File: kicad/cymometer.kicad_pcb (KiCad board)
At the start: 2 copper layers, 88.4 x 62 mm, 41 parts, among them IC1 ATTINY2313-P, P1 BNC, P2 CONN_2, P3 CONN_3X2, P4 CONN_12, Q1 BC550, U1 7805, X1 16.000

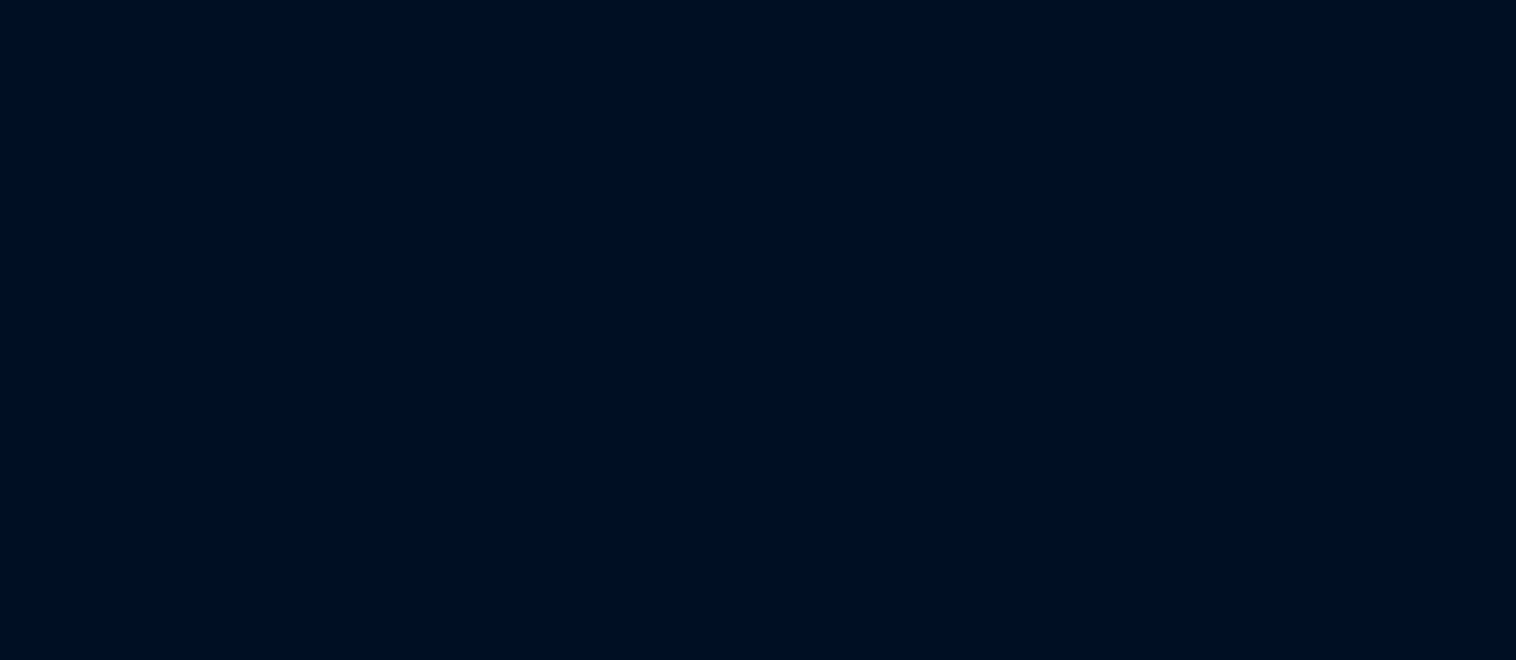
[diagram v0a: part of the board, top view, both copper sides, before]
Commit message: Add display board
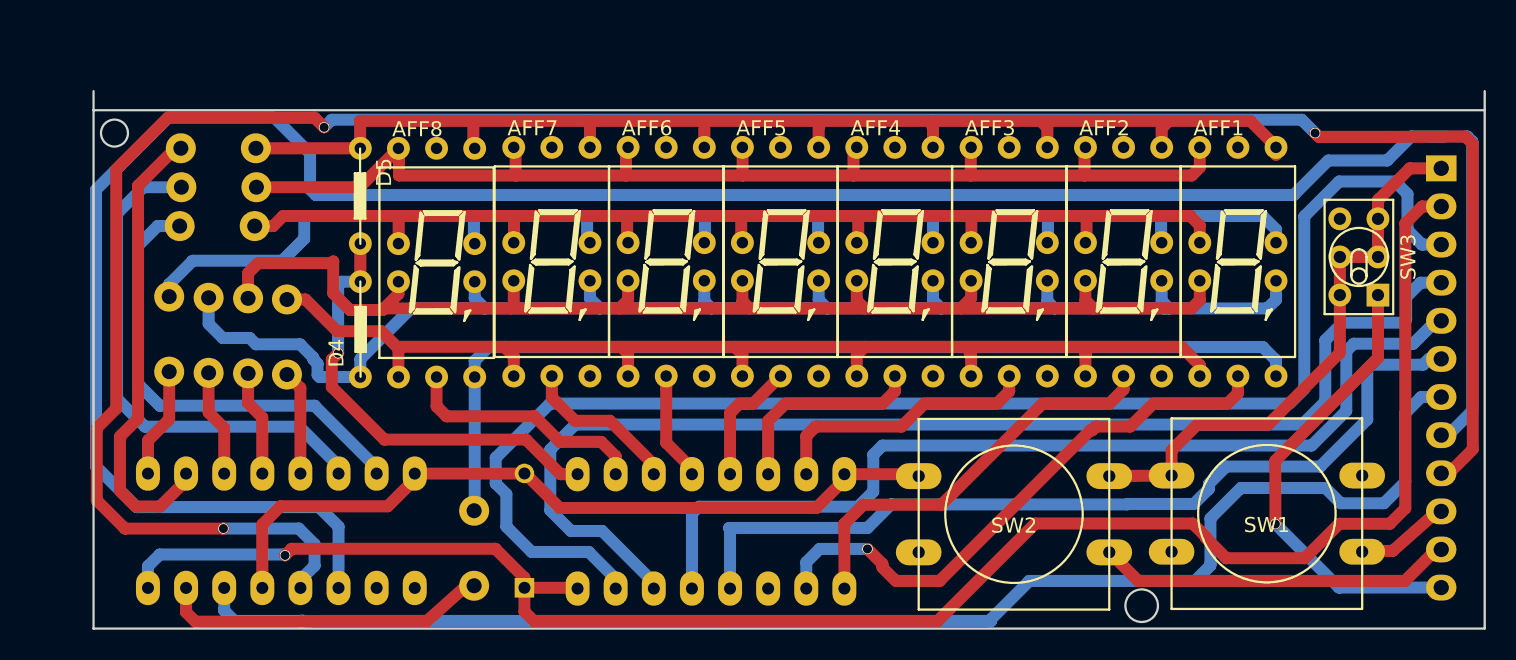
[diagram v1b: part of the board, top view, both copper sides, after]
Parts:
- added AFF1: 7SEGMENTS, cymometer:7segment_small, F.Cu at (155.0, 114.2)
- added AFF2: 7SEGMENTS, cymometer:7segment_small, F.Cu at (147.4, 114.2)
- added AFF3: 7SEGMENTS, cymometer:7segment_small, F.Cu at (139.8, 114.2)
- added AFF4: 7SEGMENTS, cymometer:7segment_small, F.Cu at (132.1, 114.2)
- added AFF5: 7SEGMENTS, cymometer:7segment_small, F.Cu at (124.5, 114.2)
- added AFF6: 7SEGMENTS, cymometer:7segment_small, F.Cu at (116.9, 114.2)
- added AFF7: 7SEGMENTS, cymometer:7segment_small, F.Cu at (109.3, 114.2)
- added AFF8: 7SEGMENTS, cymometer:7segment_small, F.Cu at (101.6, 114.3)
- added C13: C, cymometer:C_Rect_L7_W2.5_P5, B.Cu at (107.5, 132.2)
- added D4: LED, cymometer:LED, F.Cu at (96.5, 118.1)
- added D5: LED, cymometer:LED, F.Cu at (96.5, 110.5)
- added DD6: к155ид10, Housings_DIP:DIP-16_W7.62mm_LongPads, B.Cu at (111.0, 128.4)
- added DD7: 74HC595, Housings_DIP:DIP-16_W7.62mm_LongPads, B.Cu at (82.4, 128.4)
- added P5: CONN_12, Pin_Headers:Pin_Header_Straight_1x12, B.Cu at (168.6, 108.0)
- added R12: R, Resistors_ThroughHole:Resistor_Vertical_RM5mm, B.Cu at (104.1, 133.3)
- added R13: R, Resistors_ThroughHole:Resistor_Vertical_RM5mm, B.Cu at (83.8, 119.1)
- added R14: R, Resistors_ThroughHole:Resistor_Vertical_RM5mm, B.Cu at (87.1, 106.7)
- added R15: R, Resistors_ThroughHole:Resistor_Vertical_RM5mm, B.Cu at (86.4, 119.1)
- added R16: R, Resistors_ThroughHole:Resistor_Vertical_RM5mm, B.Cu at (89.0, 119.2)
- added R17: R, Resistors_ThroughHole:Resistor_Vertical_RM5mm, B.Cu at (91.6, 119.3)
- added R18: R, Resistors_ThroughHole:Resistor_Vertical_RM5mm, B.Cu at (87.1, 109.3)
- added R19: R, Resistors_ThroughHole:Resistor_Vertical_RM5mm, B.Cu at (87.0, 111.9)
- added SW1: SW_PUSH, Buttons_Switches_ThroughHole:SW_PUSH-12mm, F.Cu at (156.9, 131.0)
- added SW2: SW_PUSH, Buttons_Switches_ThroughHole:SW_PUSH-12mm, F.Cu at (140.1, 131.1)
- added SW3: SPST, Buttons_Switches_ThroughHole:SW_NKK_G1xJP, F.Cu at (163.1, 113.9)
- C10, C11, C12, C7, C8, C9: footprint capacitors:C_Rect_L7_W2.5_P5 -> cymometer:C_Rect_L7_W2.5_P5
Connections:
- R3 pad 1: Net-(C2-Pad1) -> (no net)
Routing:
- net Net-(DD7-Pad11): track 0.00 -> 160.0 mm
- net Net-(DD7-Pad12): track 0.00 -> 157.6 mm, vias 0 -> 3
- net VCC: track 352.0 -> 471.6 mm, vias 0 -> 1
- net Net-(DD7-Pad14): track 0.00 -> 94.8 mm
- net Net-(DD6-Pad15): track 0.00 -> 94.8 mm
- net Net-(AFF1-Pad4): track 0.00 -> 93.9 mm
- net Net-(AFF1-Pad7): track 0.00 -> 91.7 mm
- net GND: track 416.7 -> 506.2 mm
- net Net-(AFF1-Pad6): track 0.00 -> 86.1 mm
- net Net-(AFF1-Pad2): track 0.00 -> 84.5 mm
- net Net-(DD6-Pad14): track 0.00 -> 80.6 mm
- net Net-(AFF1-Pad9): track 0.00 -> 78.8 mm
- net Net-(AFF1-Pad10): track 0.00 -> 77.3 mm
- net Net-(AFF1-Pad1): track 0.00 -> 77.1 mm
- net Net-(AFF1-Pad5): track 0.00 -> 65.2 mm
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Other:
- board size 88.4 x 62 mm -> 143 x 118.6 mm
